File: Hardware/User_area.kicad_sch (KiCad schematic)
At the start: 0 parts

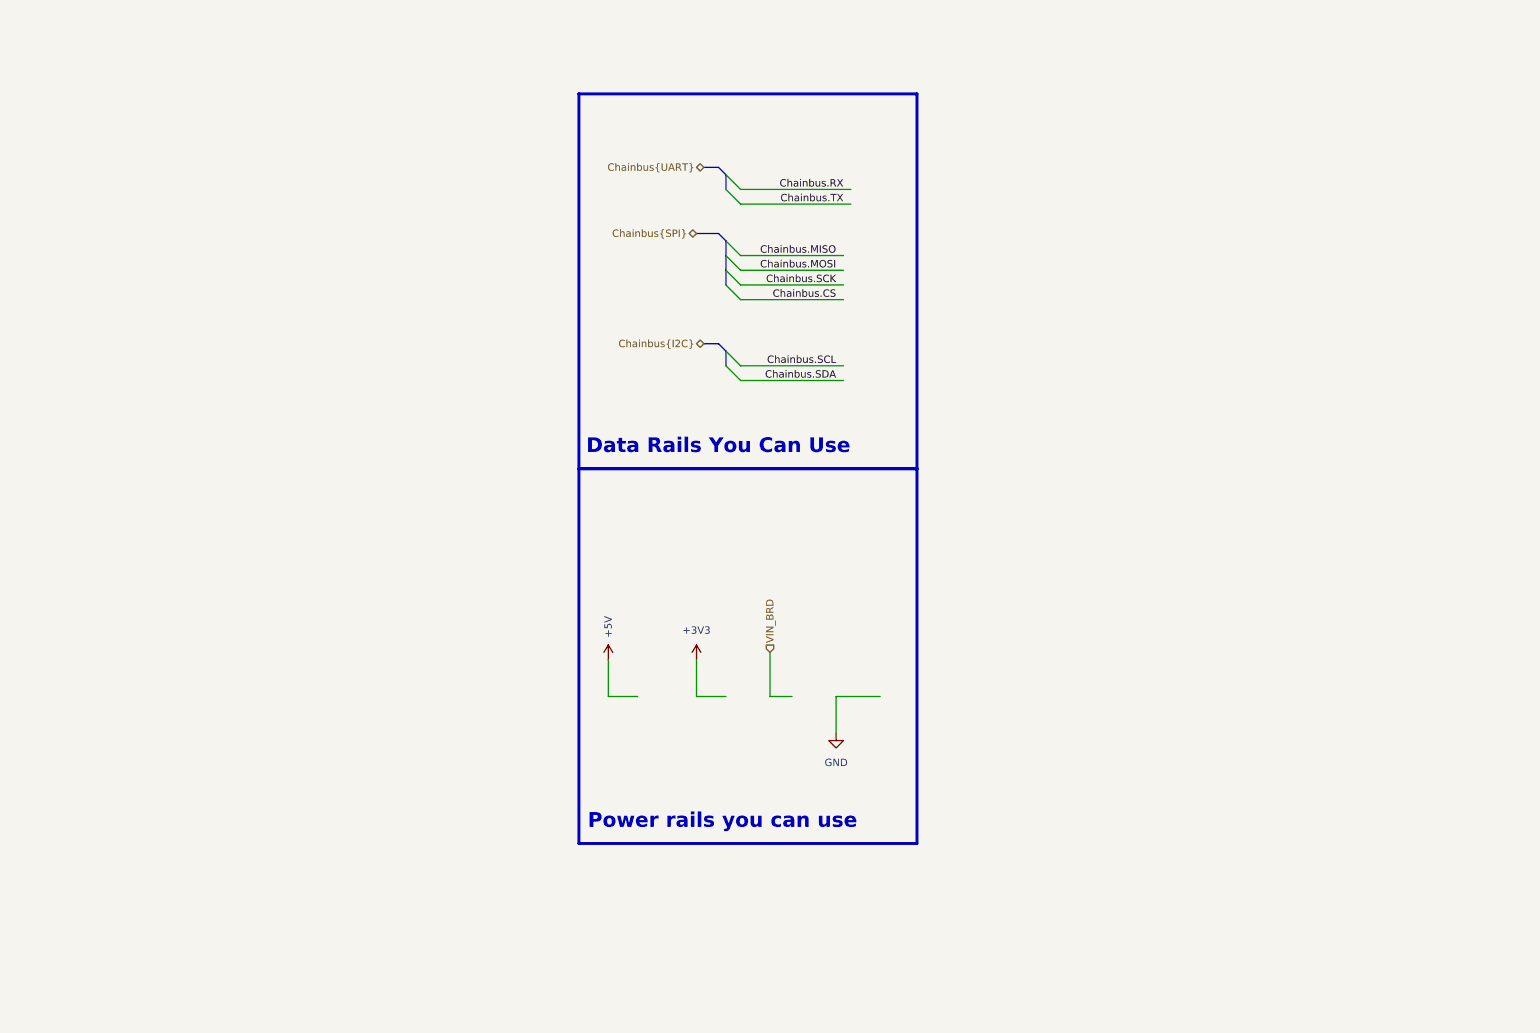
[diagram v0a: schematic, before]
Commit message: V1.0
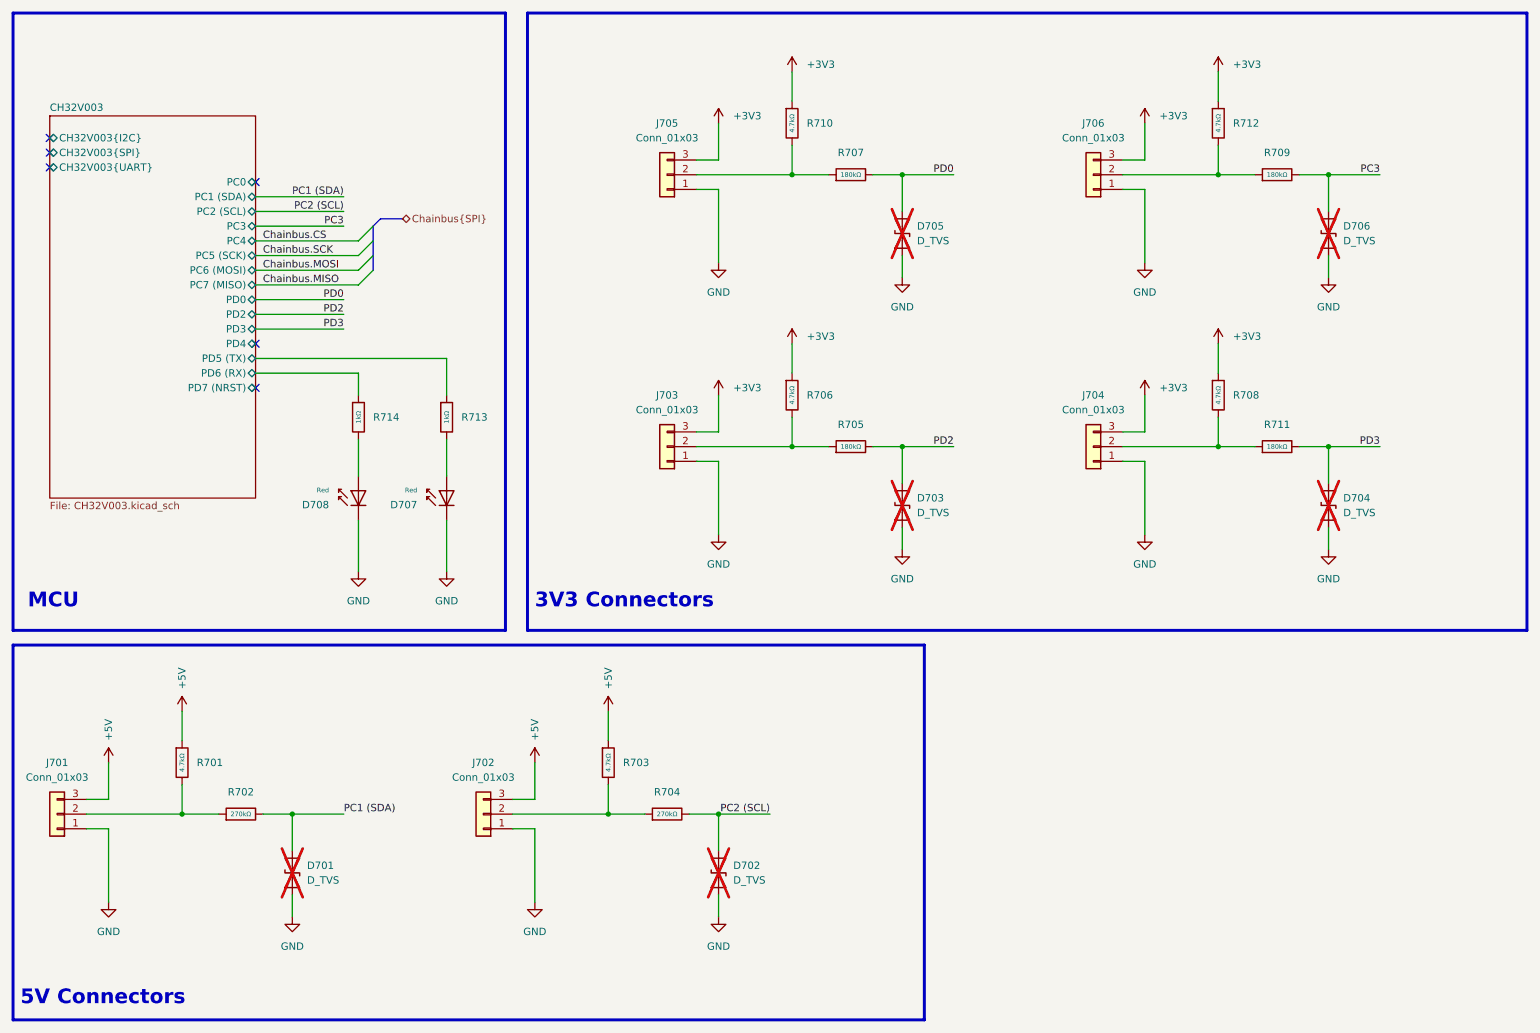
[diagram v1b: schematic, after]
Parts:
- added D701, D702, D703, D704, D705, D706: D_TVS, Diode_SMD:D_0603_1608Metric, symbol Device:D_TVS
- added D707, D708: Red, PCM_JLCPCB:D_0603, symbol PCM_JLCPCB-Diodes:LED,0603,Red
- added J701, J702, J703, J704, J705, J706: Conn_01x03, Connector_JST:JST_XH_S3B-XH-A_1x03_P2.50mm_Horizontal, symbol Connector_Generic:Conn_01x03
- added R701, R703, R706, R708, R710, R712: 4.7kΩ, PCM_JLCPCB:R_0603, symbol PCM_JLCPCB-Resistors:0603,4.7kΩ
- added R702, R704: 270kΩ, PCM_JLCPCB:R_0603, symbol PCM_JLCPCB-Resistors:0603,270kΩ
- added R705, R707, R709, R711: 180kΩ, PCM_JLCPCB:R_0603, symbol PCM_JLCPCB-Resistors:0603,180kΩ
- added R713, R714: 1kΩ, PCM_JLCPCB:R_0603, symbol PCM_JLCPCB-Resistors:0603,1kΩ
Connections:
- net +3V3: now also J703.3 (Pin_3), J704.3 (Pin_3), J705.3 (Pin_3), J706.3 (Pin_3), R706.1, R708.1, R710.1, R712.1
- net +5V: now also J701.3 (Pin_3), J702.3 (Pin_3), R701.1, R703.1
- net GND: now also D701.1 (A1), D702.1 (A1), D703.1 (A1), D704.1 (A1), D705.1 (A1), D706.1 (A1), D707.1, D708.1, J701.1 (Pin_1), J702.1 (Pin_1), J703.1 (Pin_1), J704.1 (Pin_1), J705.1 (Pin_1), J706.1 (Pin_1)
- new net: J704.2 (Pin_2), R708.2, R711.1
- new net: J702.2 (Pin_2), R703.2, R704.1
- new net: J701.2 (Pin_2), R701.2, R702.1
- new net: D707.2, R713.2
- new net: J706.2 (Pin_2), R709.1, R712.2
- new net: J705.2 (Pin_2), R707.1, R710.2
- new net: D708.2, R714.2
- new net: J703.2 (Pin_2), R705.1, R706.2
- new net CH32V003/PD5 (TX): R713.1
- new net CH32V003/PD6 (RX): R714.1
- new net PC1 (SDA): D701.2 (A2), R702.2
- new net PC2 (SCL): D702.2 (A2), R704.2
- new net PC3: D706.2 (A2), R709.2
- new net PD0: D705.2 (A2), R707.2
- new net PD2: D703.2 (A2), R705.2
- new net PD3: D704.2 (A2), R711.2
- no-connect marks 0 -> 6
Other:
- added sheet CH32V003 (CH32V003.kicad_sch)
- note added: "3V3 Connectors"
- note added: "5V Connectors"
- note added: "MCU"
- note removed: "Data Rails You Can Use"
- note removed: "Power rails you can use"
- company: (none) -> MiniModucard System
- title: (none) -> MMS3_Hat_One_Wire
